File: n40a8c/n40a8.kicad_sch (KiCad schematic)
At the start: 107 parts, among them J1 Conn_01x01_Socket, J2 Conn_01x01_Socket, J3 Conn_01x01_Socket, J4 Conn_01x01_Socket, SW1 SW_Push, SW10 SW_Push, SW11 SW_Push, SW12 SW_Push, SW13 SW_Push, SW14 SW_Push, SW15 SW_Push, SW16 SW_Push, SW17 SW_Push, SW18 SW_Push, SW19 SW_Push, SW2 SW_Push, SW20 SW_Push, SW21 SW_Push, SW22 SW_Push, SW23 SW_Push, SW24 SW_Push, SW25 SW_Push, SW26 SW_Push, SW27 SW_Push, SW28 SW_Push, SW29 SW_Push, SW3 SW_Push, SW30 SW_Push, SW31 SW_Push, SW32 SW_Push, SW33 SW_Push, SW34 SW_Push, SW35 SW_Push, SW36 SW_Push, SW37 SW_Push, SW38 SW_Push, SW39 SW_Push, SW4 SW_Push, SW40 SW_Push, SW41 SW_Push, SW42 SW_Push, SW43 SW_PWR, SW5 SW_Push, SW6 SW_Push, SW7 SW_Push, SW8 SW_Push, SW9 SW_Push, U1 XIAO-nRF52840-SMD

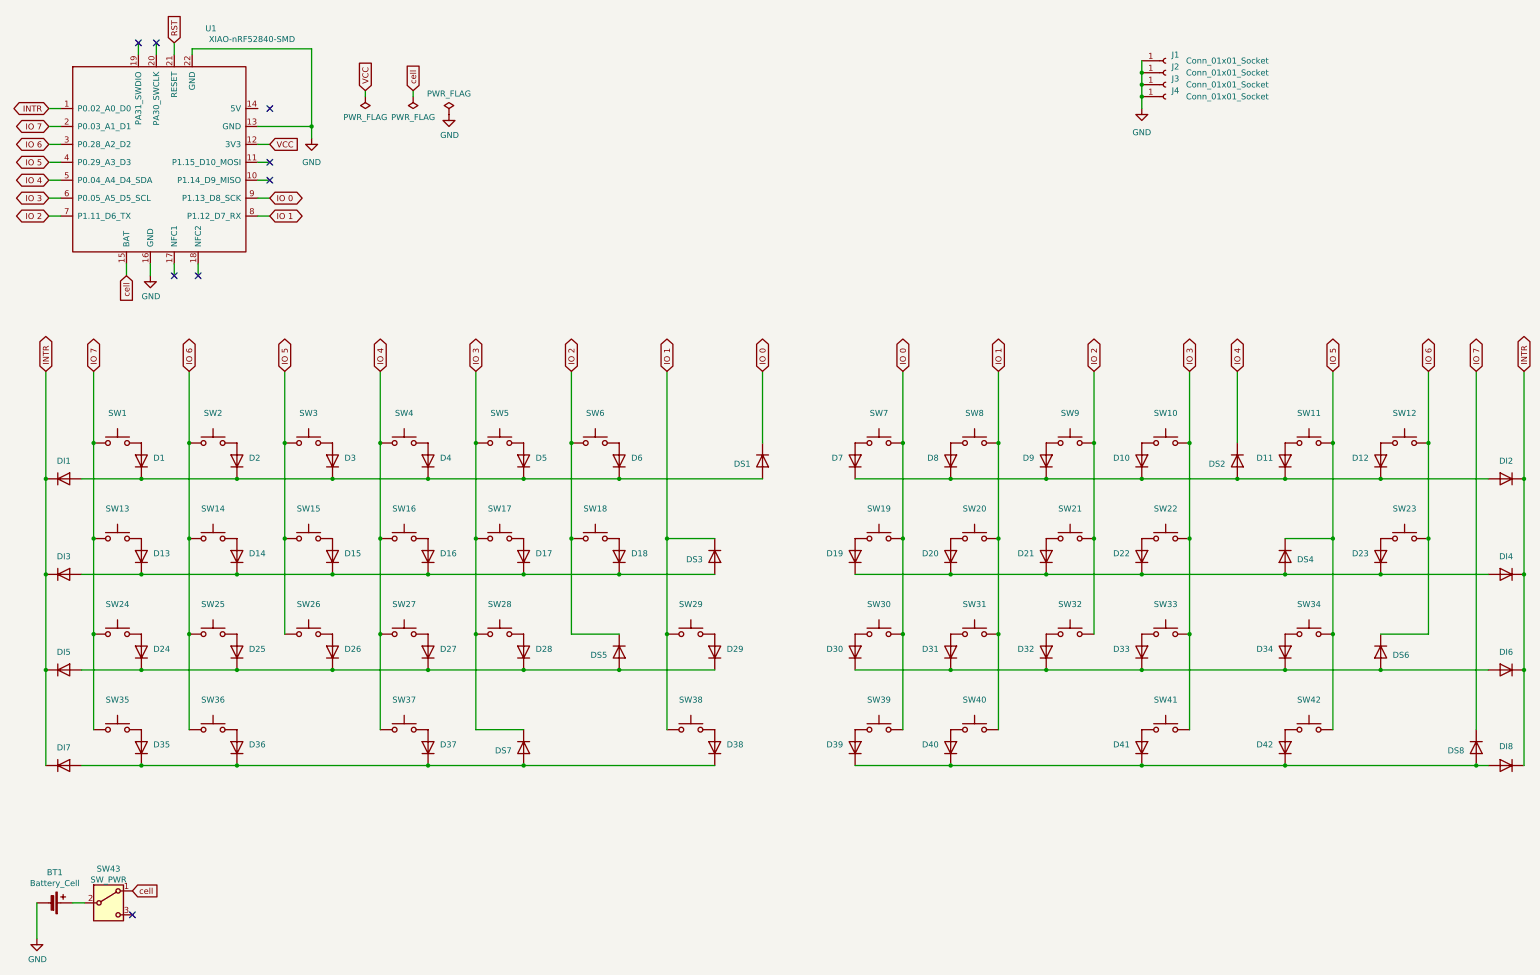
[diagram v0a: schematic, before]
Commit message: rewire
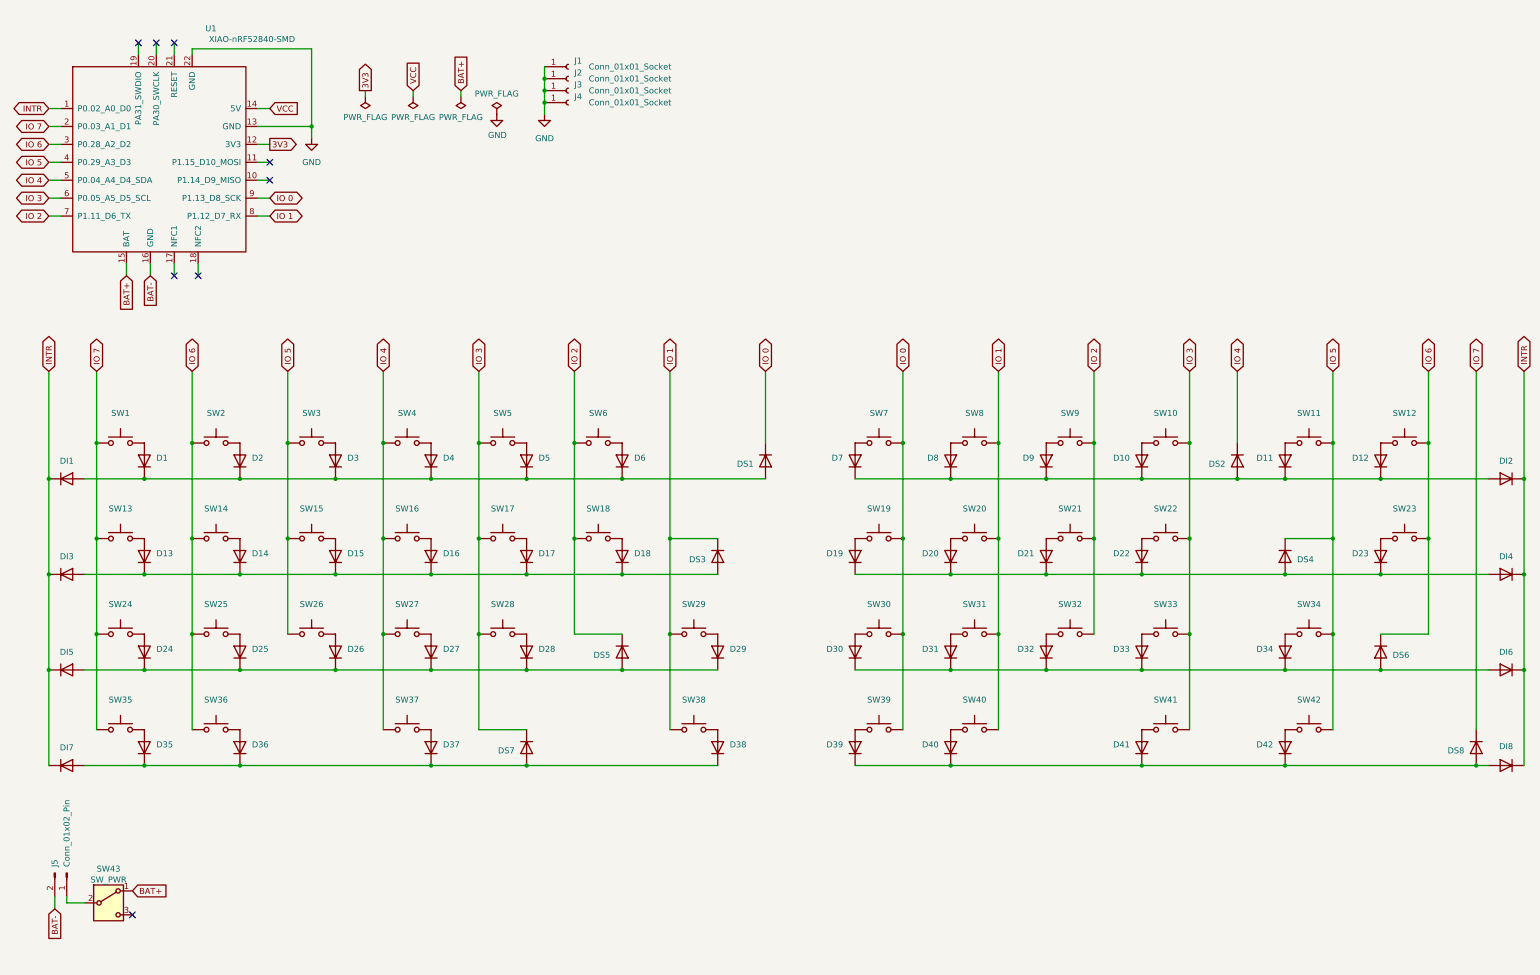
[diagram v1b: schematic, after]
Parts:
- removed BT1: Battery_Cell, Battery:BatteryHolder_Keystone_2466_1xAAA, symbol Device:Battery_Cell
- added J5: Conn_01x02_Pin, symbol Connector:Conn_01x02_Pin
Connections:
- net GND: no longer U1.16 (GND)
- net VCC: now also U1.14 (5V); no longer U1.12 (3V3)
- net at SW43.2 (B): now also J5.1 (Pin_1)
- net RST: no longer names the net of U1.21 (RESET)
- net cell renamed BAT+
- new net 3V3: U1.12 (3V3)
- new net BAT-: J5.2 (Pin_2), U1.16 (GND)
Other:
- moved on the sheet: D1, D13, D14, D15, D16, D17, D18, D2, D24, D25, D26, D27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
